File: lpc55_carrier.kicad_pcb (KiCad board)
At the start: 4 copper layers, 50 parts, among them J101 Conn_2Rows-51Pins, U101 LPC55S28JBD64, Y101 16MHz, Y102 32.768kHz

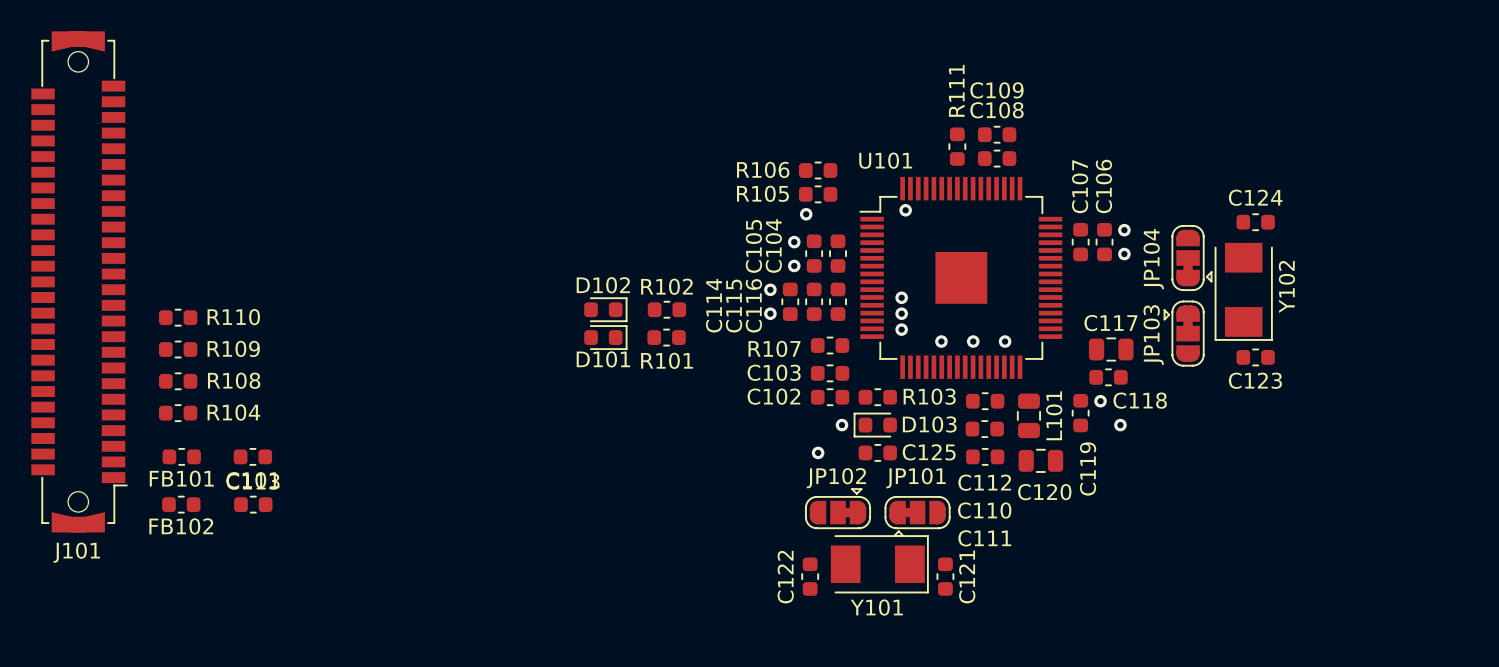
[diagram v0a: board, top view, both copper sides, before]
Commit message: lpc55_carrier: all nets routed
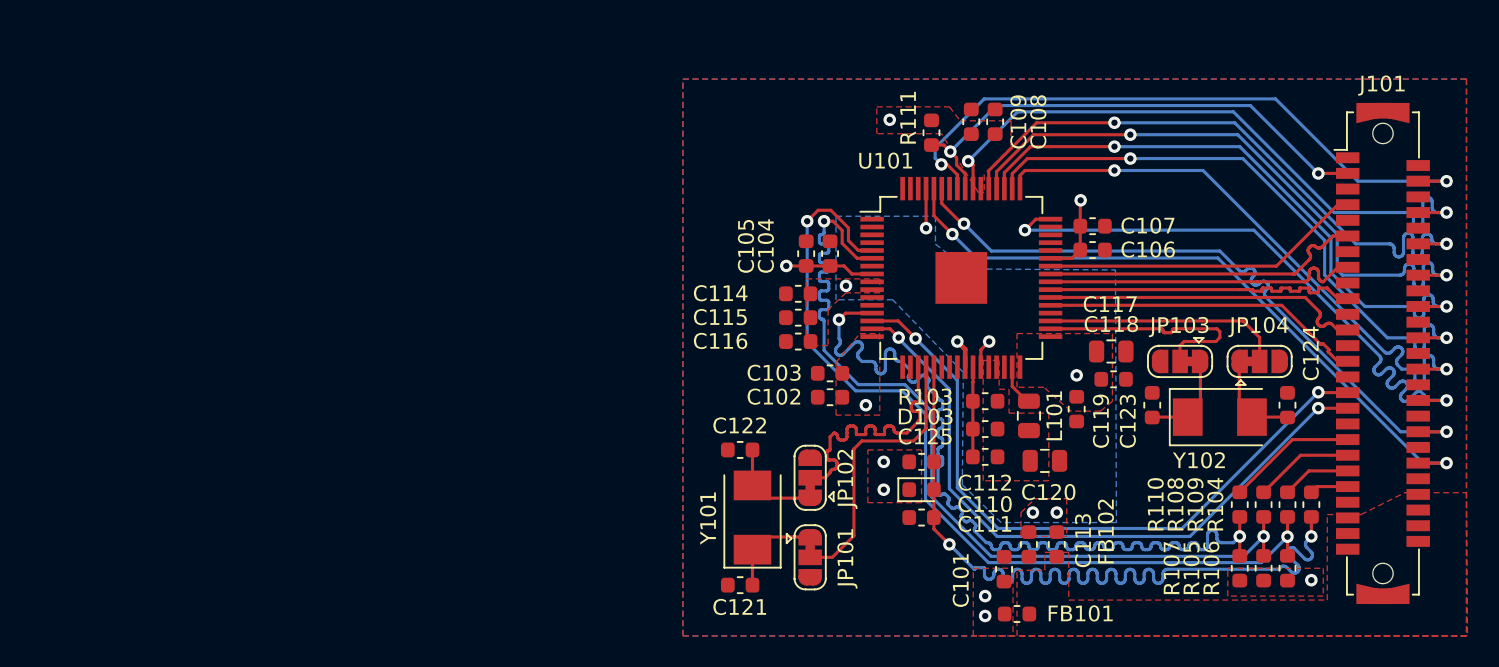
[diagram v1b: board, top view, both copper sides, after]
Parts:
- removed D101, D102: LED, LED_SMD:LED_0603_1608Metric
- removed R101, R102: 330R, Resistor_SMD:R_0603_1608Metric
- moved J101 83.4 mm to (110.7, 68.3), turned to 0 degrees
- moved R104 72.6 mm to (106.2, 78.0), turned to 90 degrees
- moved R109 71.5 mm to (104.6, 78.0), turned to 90 degrees
- moved R108 69.8 mm to (103.1, 78.0), turned to 90 degrees
- moved R110 68.8 mm to (101.6, 78.0), turned to 90 degrees
- moved FB102 56.0 mm to (89.9, 80.5), turned to 270 degrees
- moved FB101 54.3 mm to (87.4, 85.0), turned to 0 degrees
- moved C113 49.6 mm to (88.1, 80.5), turned to 270 degrees
- moved C101 48.5 mm to (86.6, 82.1), turned to 90 degrees
- moved R106 39.3 mm to (104.6, 82.0), turned to 90 degrees
- moved R105 37.1 mm to (103.1, 82.0), turned to 90 degrees
- moved R107 29.8 mm to (101.6, 82.0), turned to 90 degrees
- moved C121 13.1 mm to (69.7, 83.1), turned to 180 degrees
- moved C124 11.9 mm to (104.6, 71.6), turned to 90 degrees
- moved C122 9.24 mm to (69.7, 74.5), turned to 180 degrees
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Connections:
- J101 pad 1: +3V3 -> GND
- J101 pad 11: GND -> /HS_SPI_SCK
- J101 pad 12: /FC3_CTS_SDAX_SSEL0 -> /FC3_RXD_DSA_MOSI
- J101 pad 13: /SWD_CLK -> GND
- J101 pad 15: GND -> /HS_SPI_MOSI
- J101 pad 16: /FC3_RTS_SCLX_SSEL1 -> /FC3_TXD_SCL_MISO
- J101 pad 17: /SWD_IO -> GND
- J101 pad 19: GND -> /~HS_SPI_SSEL1
- J101 pad 2: +3V3 -> GND
- J101 pad 20: /PIO0_22 -> /PIO0_25
- J101 pad 21: /SWD_TRACESWO -> GND
- J101 pad 23: GND -> /~HS_SPI_IRQ
- J101 pad 24: /PIO0_25 -> /PIO0_22
- J101 pad 25: /ISP0 -> GND
- J101 pad 27: GND -> /~SP_RESET
- J101 pad 28: /FC3_TXD_SCL_MISO -> /FC3_RTS_SCLX_SSEL1
- J101 pad 29: /HS_SPI_SCK -> GND
- J101 pad 3: +3V3 -> /ISP0
- J101 pad 31: GND -> /SCT0_OUT2
- J101 pad 32: /FC3_RXD_DSA_MOSI -> /FC3_CTS_SDAX_SSEL0
- J101 pad 33: /HS_SPI_MISO -> /SCT0_OUT3
- J101 pad 36: /PIO0_4 -> /FC0_RXD
- J101 pad 37: /HS_SPI_MOSI -> /SWD_TRACESWO
- J101 pad 39: GND -> /SWD_CLK
- J101 pad 4: +3V3 -> /FC3_SCK
- J101 pad 40: /FC3_SCK -> /FC0_TXD
- J101 pad 41: /~HS_SPI_SSEL1 -> /SWD_IO
- J101 pad 43: GND -> /~SWD_RESET
- J101 pad 44: /FC0_RXD -> +3V3
- J101 pad 45: /~HS_SPI_IRQ -> GND
- J101 pad 46: GND -> +3V3
- J101 pad 47: GND -> +3V3
- J101 pad 48: /FC0_TXD -> +3V3
- J101 pad 49: /~SP_RESET -> +3V3
- J101 pad 5: +3V3 -> GND
- J101 pad 50: GND -> +3V3
- J101 pad 51: GND -> +3V3
- J101 pad 6: +3V3 -> GND
- J101 pad 7: GND -> /HS_SPI_MISO
- J101 pad 8: +3V3 -> /PIO0_4
- J101 pad 9: /~SWD_RESET -> GND
- JP101 pad 2: (no net) -> /OSC_IN
- JP102 pad 2: (no net) -> /OSC_OUT
- JP103 pad 2: (no net) -> /OSC_RTC_IN
- JP104 pad 2: (no net) -> /OSC_RTC_OUT
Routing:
- net /PIO0_10: track 0.00 -> 56.7 mm, vias 0 -> 2
- net /PIO0_11: track 0.00 -> 56.6 mm, vias 0 -> 2
- net /PIO0_12: track 0.00 -> 56.6 mm, vias 0 -> 2
- net /~RESET: track 0.00 -> 54.0 mm, vias 0 -> 2
- net /SCT0_OUT2: track 0.00 -> 43.5 mm, vias 1 -> 2
- net /SCT0_OUT3: track 0.00 -> 43.0 mm, vias 1 -> 2
- net /FC0_RXD: track 0.00 -> 42.9 mm, vias 0 -> 2
- net /FC0_TXD: track 0.00 -> 42.8 mm, vias 0 -> 2
- net /FC3_RXD_DSA_MOSI: track 0.00 -> 41.4 mm, vias 0 -> 2
- net /FC3_CTS_SDAX_SSEL0: track 0.00 -> 41.4 mm, vias 0 -> 2
- net /FC3_SCK: track 0.00 -> 41.3 mm, vias 0 -> 2
- net /FC3_TXD_SCL_MISO: track 0.00 -> 41.3 mm, vias 0 -> 2
- net /PIO0_4: track 0.00 -> 41.3 mm, vias 0 -> 2
- net /FC3_RTS_SCLX_SSEL1: track 0.00 -> 39.6 mm, vias 0 -> 2
- net /PIO0_22: track 0.00 -> 39.5 mm, vias 0 -> 2
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- added copper zone on F.Cu, net +3V3
- added copper zone on F.Cu, net /FB
- added copper zone on B.Cu, net /VDD
- added copper zone on F.Cu, net /VDD
- added copper zone on B.Cu, net /VDDA
- added copper zone on F.Cu, net /VDDA
- added copper zone on F.Cu, net GND
